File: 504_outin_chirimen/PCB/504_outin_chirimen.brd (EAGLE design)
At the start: 48 x 80 mm, 19 parts

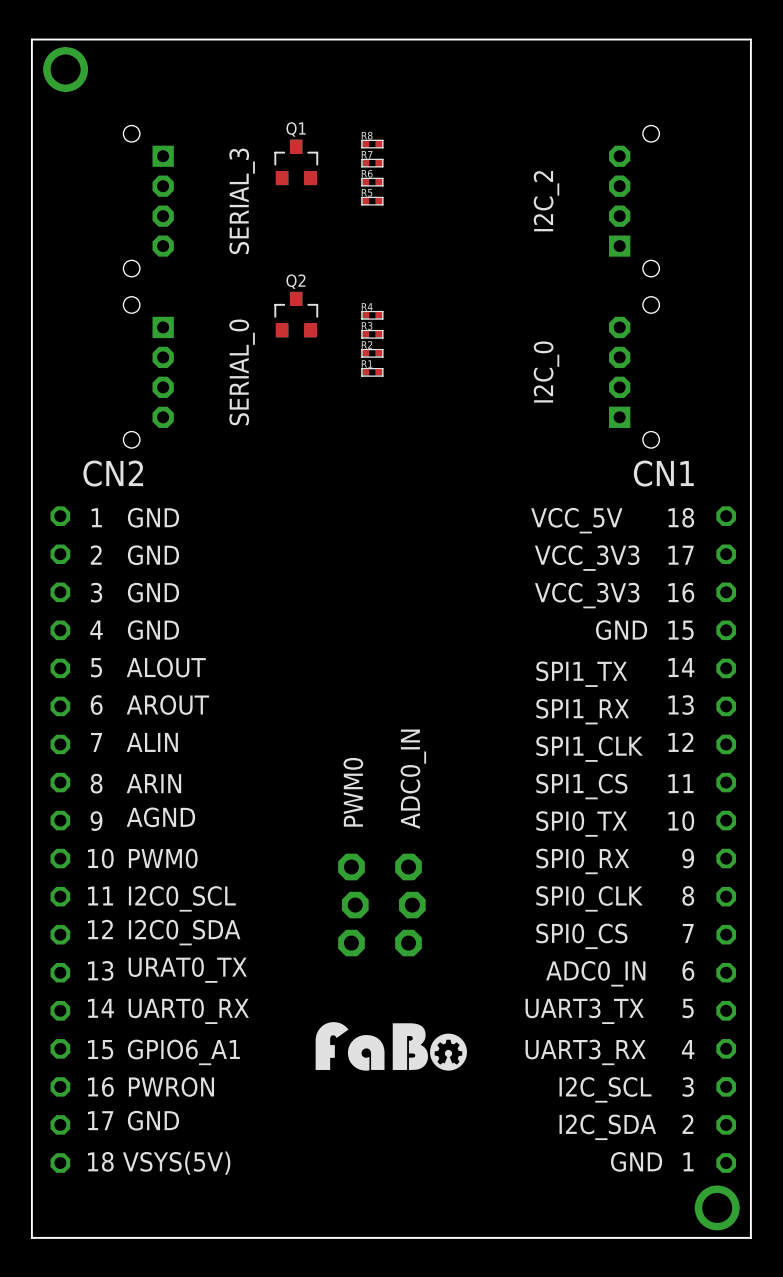
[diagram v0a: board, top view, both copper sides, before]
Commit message: Update chirimen
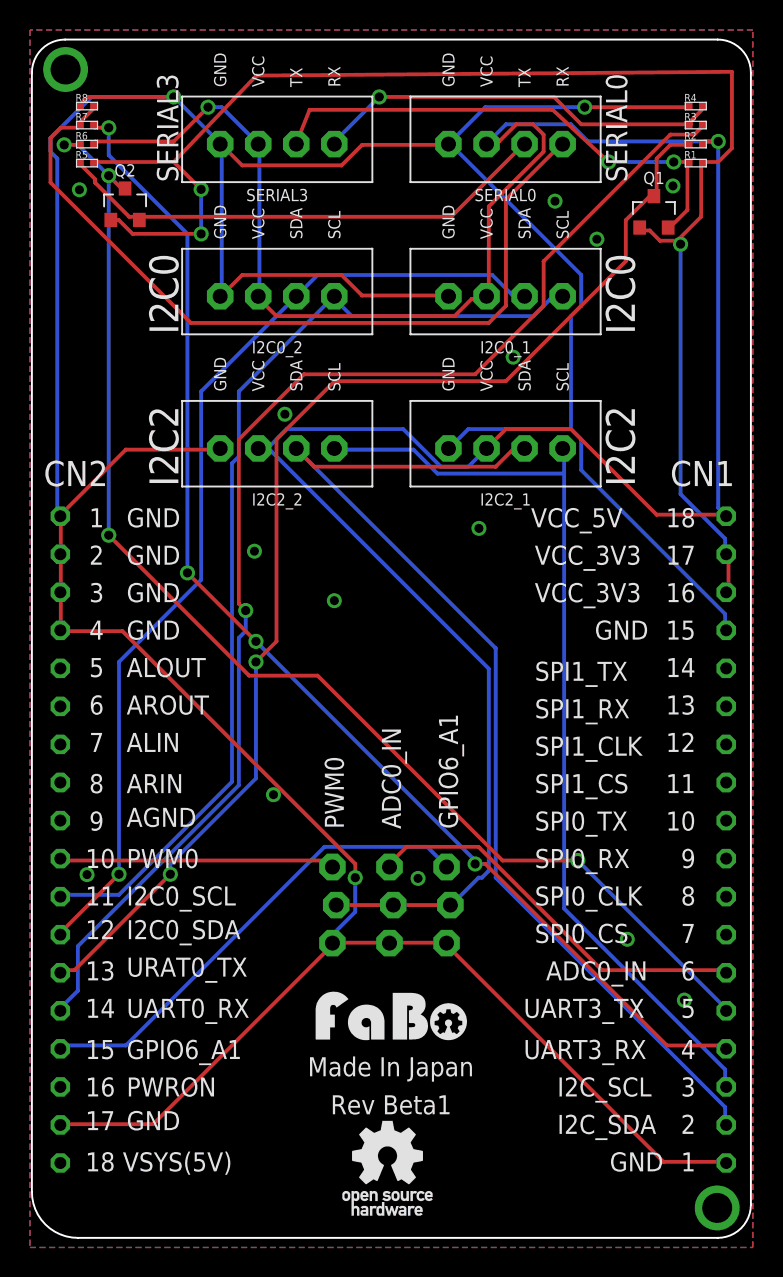
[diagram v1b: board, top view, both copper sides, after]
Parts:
- removed I2C_0, I2C_2: (no value), FaBo-Template:FABO_BRICK_I2C_S04B-PASK-2
- removed SERIAL_0, SERIAL_3: (no value), FaBo-Template:FABO_BRICK_SERIAL_S04B-PASK-2
- removed U$22: (no value), FaBo-etc:LOGO_OSHW_T_MS_BOTTOM
- added GPIO6_A1: (no value), FaBo-Template:FABO_BRICK_3PIN_HEADER
- added I2C0_1, I2C0_2, I2C2_1, I2C2_2: (no value), FaBo-Template:FABO_BRICK_I2C_CONNECTOR_I_SILK
- added SERIAL0, SERIAL3: (no value), FaBo-Template:FABO_BRICK_SERIAL_CONNECTOR_I_SILK
- added U$3: (no value), FaBo-etc:LOGO_OSHW_T_M
- moved R3 25.7 mm to (44.5, 74.9)
- moved R4 25.7 mm to (44.5, 76.2)
- moved R1 25.7 mm to (44.5, 72.4)
- moved R2 25.7 mm to (44.5, 73.7)
- moved Q1 24.1 mm to (41.7, 69.1)
- moved R5 19.2 mm to (3.81, 72.4)
- moved R7 19.2 mm to (3.81, 74.9)
- moved R8 19.2 mm to (3.81, 76.2)
- moved R6 19.2 mm to (3.81, 73.7)
- moved Q2 13.6 mm to (6.35, 69.6)
- moved U$10 2.03 mm to (24.1, 13.5)
- moved ADC0_IN 1.27 mm to (24.1, 22.9)
- moved PWM0 1.27 mm to (20.3, 22.9)
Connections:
- new net GPIO6_A1: GPIO6_A1.I/O, U$2.CN2_15
- net 5V: now also GPIO6_A1.VCC, I2C0_1.VCC, I2C0_2.VCC, I2C2_1.VCC, I2C2_2.VCC, SERIAL0.VCC, SERIAL3.VCC; no longer I2C_0.VCC, I2C_2.VCC, SERIAL_0.VCC, SERIAL_3.VCC
- net GND: now also GPIO6_A1.GND, I2C0_1.GND, I2C0_2.GND, I2C2_1.GND, I2C2_2.GND, SERIAL0.GND, SERIAL3.GND, U$2.CN1_15; no longer I2C_0.GND, I2C_2.GND, SERIAL_0.GND, SERIAL_3.GND
- net RX0: now also SERIAL3.RX; no longer SERIAL_3.RX
- net RX3: now also SERIAL0.RX; no longer SERIAL_0.RX
- net SCL0: now also I2C0_1.SCL, I2C0_2.SCL; no longer I2C_2.SCL
- net SCL2: now also I2C2_1.SCL, I2C2_2.SCL; no longer I2C_0.SCL
- net SDA0: now also I2C0_1.SDA, I2C0_2.SDA; no longer I2C_2.SDA
- net SDA2: now also I2C2_1.SDA, I2C2_2.SDA; no longer I2C_0.SDA
- net TX0: now also SERIAL3.TX; no longer SERIAL_3.TX
- net TX3: now also SERIAL0.TX; no longer SERIAL_0.TX
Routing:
- net GND: track 0.00 -> 263.6 mm, vias 0 -> 17
- net 5V: track 0.00 -> 182.2 mm, vias 0 -> 2
- net 3V3: track 0.00 -> 98.2 mm, vias 0 -> 3
- net UART0_RX: track 0.00 -> 84.9 mm, vias 0 -> 1
- net UART3_TX: track 0.00 -> 84.8 mm, vias 0 -> 4
- net UART3_RX: track 0.00 -> 82.3 mm, vias 0 -> 4
- net UART0_TX: track 0.00 -> 81.0 mm, vias 0 -> 2
- net SDA2: track 0.00 -> 73.3 mm
- net SCL0: track 0.00 -> 66.4 mm
- net SDA0: track 0.00 -> 65.5 mm, vias 0 -> 1
- net SCL2: track 0.00 -> 63.2 mm
- net RX3: track 0.00 -> 54.2 mm
- net TX0: track 0.00 -> 34.1 mm, vias 0 -> 2
- net TX3: track 0.00 -> 33.6 mm
- net GPIO6_A1: track 0.00 -> 32.1 mm
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- added copper zone on layer 1, net GND
- added copper zone on layer 16, net GND
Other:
- outline, holes or cut-outs redrawn
- board text added: "I2C0"
- board text added: "I2C2"
- board text added: "Made In Japan"
- board text added: "Rev Beta1"
- board text added: "SERIAL0"
- board text added: "SERIAL3"
